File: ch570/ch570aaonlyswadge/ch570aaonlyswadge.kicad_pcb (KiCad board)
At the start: 2 copper layers, 42 x 26.8 mm, 53 parts, among them J1 SAO, J2 USB_C_Receptacle_USB2.0_16P, SW2 TS-1187A-B-A-B, U1 CH572D, U2 AW32001, U3 QMC6309, U4 USBLC6-2SC6, U7 MG6229D4-28, Y1 32MHz

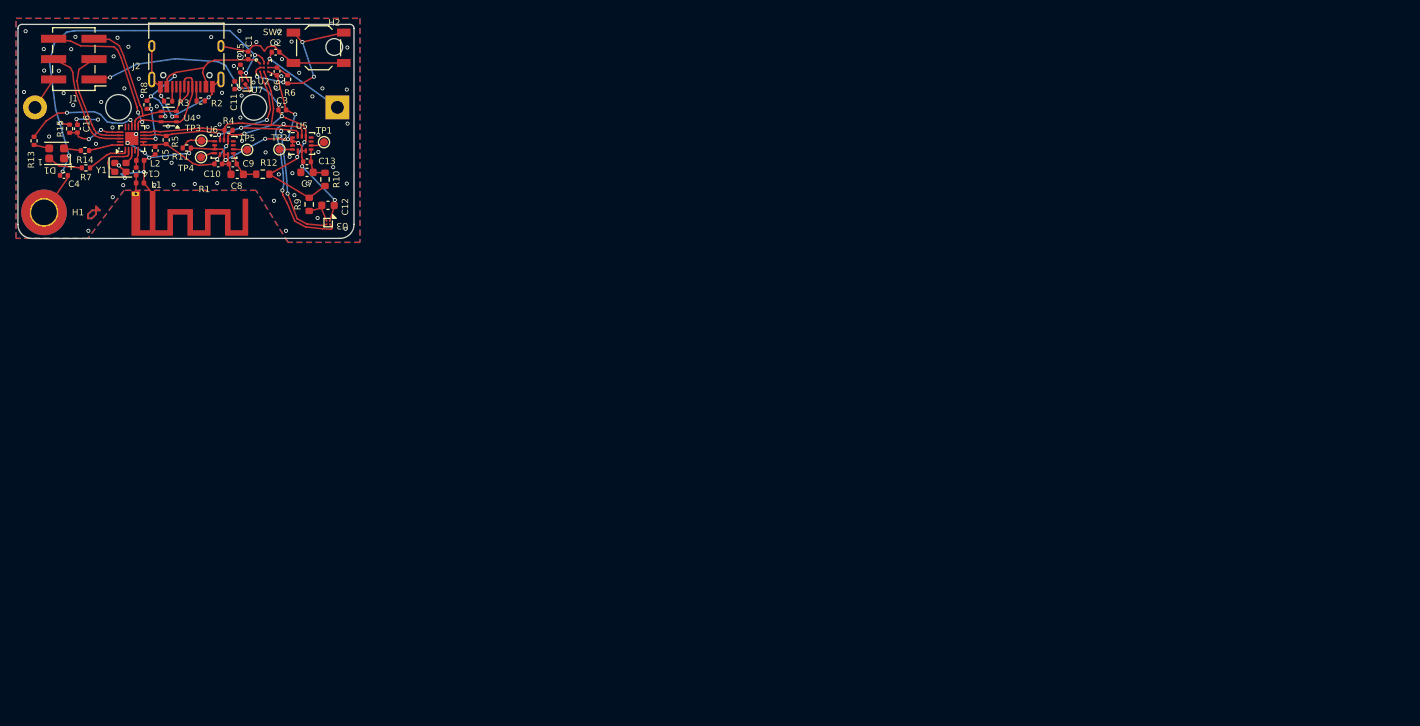
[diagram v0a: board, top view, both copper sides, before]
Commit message: Bump aa swadge
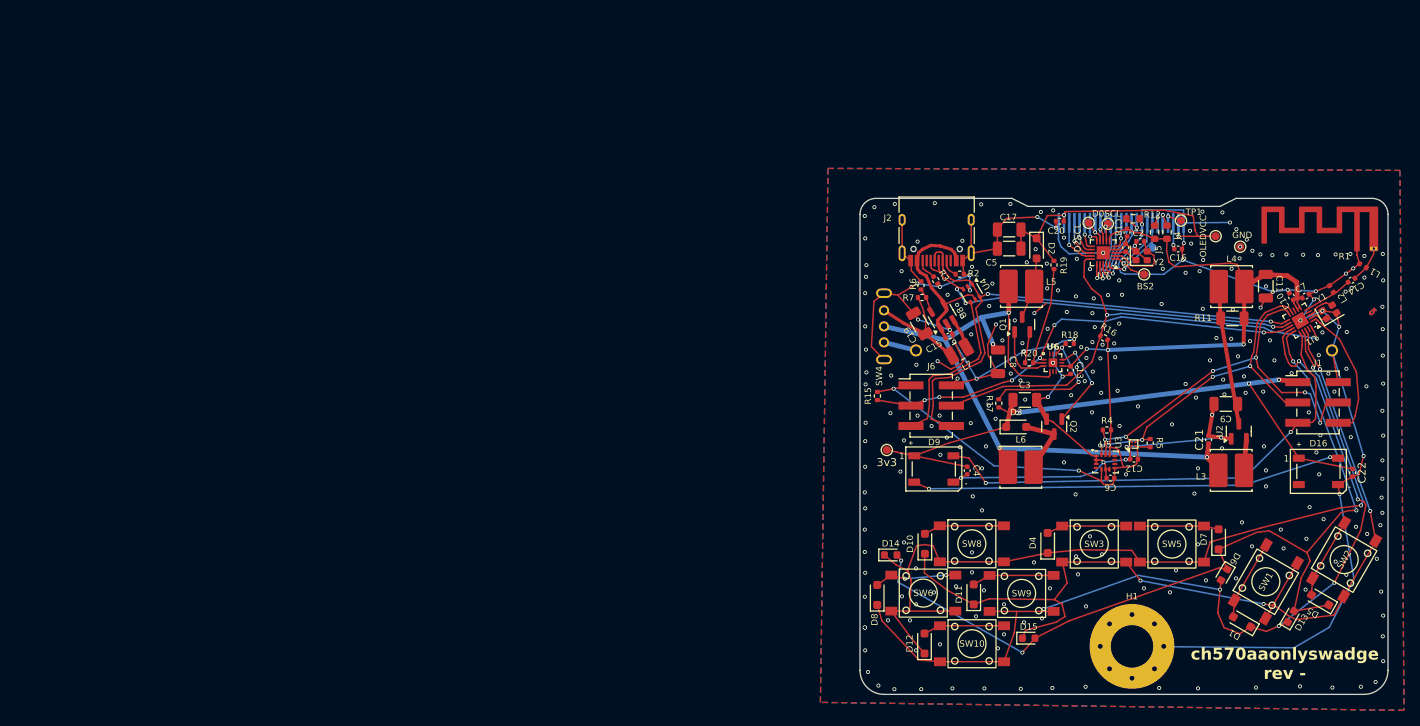
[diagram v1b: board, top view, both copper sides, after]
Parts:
- removed H2: BATTMOUNT, MountingHole:MountingHole_2.1mm
- removed R10, R9: 33Ω, Resistor_SMD:R_0603_1608Metric
- removed R13, R14: 1k, Resistor_SMD:R_0402_1005Metric
- removed R8: NP, Resistor_SMD:R_0402_1005Metric
- added C17: 22u25v-BASIC, Capacitor_SMD:C_1206_3216Metric, F.Cu at (187.7, 59.9)
- added C18: 1u, Capacitor_SMD:C_0402_1005Metric, F.Cu at (202.4, 60.3)
- added C19: 22u25v-BASIC, Capacitor_SMD:C_1206_3216Metric, F.Cu at (176.4, 71.6)
- added C20: 1u, Capacitor_SMD:C_0402_1005Metric, F.Cu at (194.0, 58.9)
- added C21: 1u, Capacitor_SMD:C_0402_1005Metric, F.Cu at (212.6, 86.2)
- added C22: 1u, Capacitor_SMD:C_0402_1005Metric, F.Cu at (230.6, 90.3)
- added D10: 1N4148WS, Diode_SMD:D_SOD-323_HandSoldering, F.Cu at (177.1, 99.2)
- added D11: 1N4148WS, Diode_SMD:D_SOD-323_HandSoldering, F.Cu at (183.2, 105.5)
- added D12: 1N4148WS, Diode_SMD:D_SOD-323_HandSoldering, F.Cu at (177.1, 111.6)
- added D13: RED, LED_SMD:LED_0603_1608Metric, F.Cu at (222.9, 108.3)
- added D14: RED, LED_SMD:LED_0603_1608Metric, F.Cu at (172.8, 100.6)
- added D15: RED, LED_SMD:LED_0603_1608Metric, F.Cu at (190.1, 111.0)
- added D16: WS2812B, LED_SMD:LED_WS2812B_PLCC4_5.0x5.0mm_P3.2mm, F.Cu at (226.3, 90.1)
- added D2: 1A-600mV, Diode_SMD:D_SOD-323_HandSoldering, F.Cu at (191.1, 62.2)
- added D3: 1A-600mV, Diode_SMD:D_SOD-323_HandSoldering, F.Cu at (188.5, 84.6)
- added D4: 1N4148WS, Diode_SMD:D_SOD-323_HandSoldering, F.Cu at (192.5, 99.1)
- added D5: 1N4148WS, Diode_SMD:D_SOD-323_HandSoldering, F.Cu at (226.5, 106.2)
- added D6: RED, LED_SMD:LED_0603_1608Metric, F.Cu at (214.5, 103.0)
- added D7: 1N4148WS, Diode_SMD:D_SOD-323_HandSoldering, F.Cu at (213.8, 98.6)
- added D8: 1N4148WS, Diode_SMD:D_SOD-323_HandSoldering, F.Cu at (171.2, 105.6)
- added D9: WS2812B, LED_SMD:LED_WS2812B_PLCC4_5.0x5.0mm_P3.2mm, F.Cu at (178.2, 89.8)
- added J3: OLED, cnhardware:RONBOE-OLED-25, B.Cu at (202.0, 59.1)
- added J4: J, Resistor_SMD:R_0603_1608Metric, F.Cu at (207.4, 60.2)
- added J5: J, Resistor_SMD:R_0603_1608Metric, F.Cu at (205.8, 60.2)
- added J6: PGM, Connector_PinHeader_2.54mm:PinHeader_2x03_P2.54mm_Vertical_SMD, F.Cu at (177.9, 81.9)
- added L3: 47uH 750mA 580mΩ, Inductor_SMD:L_Cenker_CKCS5020, F.Cu at (215.4, 90.0)
- added L4: 47uH 750mA 580mΩ, Inductor_SMD:L_Cenker_CKCS5020, F.Cu at (215.4, 67.0)
- added L5: 47uH 580mΩ, Inductor_SMD:L_Cenker_CKCS5020, F.Cu at (189.2, 67.0)
- added L6: 47uH 580mΩ, Inductor_SMD:L_Cenker_CKCS5020, F.Cu at (189.1, 89.6)
- added L7: 2.2uH, Inductor_SMD:L_1008_2520Metric, F.Cu at (181.3, 75.1)
- added Q1: 2300A, Package_TO_SOT_SMD:SOT-23, F.Cu at (189.3, 71.8)
- added Q2: 2300A, Package_TO_SOT_SMD:SOT-23, F.Cu at (193.3, 84.5)
- added R16: 5.1k, Resistor_SMD:R_0402_1005Metric, F.Cu at (199.5, 73.4)
- added R17: 5.1k, Resistor_SMD:R_0402_1005Metric, F.Cu at (186.3, 81.6)
- added R18: 5.1k, Resistor_SMD:R_0402_1005Metric, F.Cu at (195.2, 74.2)
- added R19: 51k, Resistor_SMD:R_0402_1005Metric, F.Cu at (193.2, 64.3)
- added R20: 5.1k, Resistor_SMD:R_0402_1005Metric, F.Cu at (190.1, 76.5)
- added SW1: YTS-D003-1A, cnhardware:YTS-D003-1A, F.Cu at (219.7, 103.9)
- added SW10: YTS-D003-1A, cnhardware:YTS-D003-1A, F.Cu at (183.0, 111.7)
- added SW3: YTS-D003-1A, cnhardware:YTS-D003-1A, F.Cu at (198.3, 99.2)
- added SW4: SW_SPDT_1825232-1, cnhardware:1825232-1, F.Cu at (172.0, 72.0)
- added SW5: YTS-D003-1A, cnhardware:YTS-D003-1A, F.Cu at (208.0, 99.2)
- added SW6: YTS-D003-1A, cnhardware:YTS-D003-1A, F.Cu at (176.9, 105.3)
- added SW8: YTS-D003-1A, cnhardware:YTS-D003-1A, F.Cu at (183.0, 99.2)
- added SW9: YTS-D003-1A, cnhardware:YTS-D003-1A, F.Cu at (189.2, 105.4)
- added TP6: OLEDVCC, TestPoint:TestPoint_Pad_D1.0mm, F.Cu at (213.4, 60.7)
- added TP7: GND, TestPoint:TestPoint_Pad_D1.0mm, F.Cu at (216.5, 62.0)
- added TP8: 3v3, TestPoint:TestPoint_Pad_D1.0mm, F.Cu at (172.3, 87.5)
- added U8: HX3406, Package_TO_SOT_SMD:SOT-23-5, F.Cu at (179.3, 70.7)
- added Y2: 24MHz, Crystal:Crystal_SMD_2016-4Pin_2.0x1.6mm, F.Cu at (204.2, 63.2)
- BT1: footprint Battery:BatteryHolder_Bulgin_BX0123_1xCR123 -> cnhardware:2460
- C1, C2: value 4.7u -> 10p
- C10, C13: value 0.1μF -> 1u
- C11, C9: value 0.1μF -> 100uF6.3v; footprint Capacitor_SMD:C_0402_1005Metric -> Capacitor_SMD:C_1206_3216Metric
- C12, C7: value 22μF -> 1u; footprint Capacitor_SMD:C_0603_1608Metric -> Capacitor_SMD:C_0402_1005Metric
- C15: value 1u -> 4.7u
- C16: value 0.1u -> 4.7u
- C3: value 4.7u -> 100uF6.3v; footprint Capacitor_SMD:C_0402_1005Metric -> Capacitor_SMD:C_1206_3216Metric
- C4: value 0.1u -> 1u
- C5: value 0.1u -> 22u25v-BASIC; footprint Capacitor_SMD:C_0402_1005Metric -> Capacitor_SMD:C_1206_3216Metric
- C8: value 22μF -> 100uF6.3v; footprint Capacitor_SMD:C_0603_1608Metric -> Capacitor_SMD:C_1206_3216Metric
- D1: value A-SP1923XR6GHB1C-M01-3T -> 1N4148WS; footprint LED_SMD:LED_RGB_Wuerth_150080M153000 -> Diode_SMD:D_SOD-323_HandSoldering
- H1: footprint MountingHole:MountingHole_3.2mm_M3_ISO7380_Pad_TopBottom -> MountingHole:MountingHole_5.3mm_M5_Pad_Via
- R11: value 5.1k -> J1; footprint Resistor_SMD:R_0402_1005Metric -> Resistor_SMD:R_1206_3216Metric
- R12: value 33Ω -> 1M
- R7: value 1k -> 5.1k
- SW2: value TS-1187A-B-A-B -> YTS-D003-1A; footprint Button_Switch_SMD:SW_SPST_TL3342 -> cnhardware:YTS-D003-1A
- TP1: value INT2 -> OLEDGPIO
- TP2: value INT1 -> BS1; moved to B.Cu
- TP3: value SA0 -> BS2
- TP4: value INT1 -> D0SCL
- TP5: value INT1 -> D2SCL
- U2: value AW32001 -> GR2188A22; footprint cnhardware:WLCSP-9-P0.5mm -> Package_TO_SOT_SMD:SOT-23
- U6: value ~ -> CH32V005D6U6; footprint cnhardware:LGA-14_3x2.5mm_P0.5mm_LayoutBorder3x4y_EVEN_PADS -> cnhardware:QFN-12-P0.4-WCH
- U7: value MG6229D4-28 -> CH32V006F8U6; footprint cnhardware:xdfn-reg -> Package_DFN_QFN:QFN-20-1EP_3x3mm_P0.4mm_EP1.65x1.65mm
- moved J1 161.3 mm to (226.2, 81.5), turned to 0 degrees
- moved D1 159.3 mm to (216.7, 108.9), turned to 150 degrees
- moved L1 153.2 mm to (231.9, 64.4), turned to 150 degrees
- moved C14 152.5 mm to (230.4, 66.2), turned to -150 degrees
- moved Y1 152.2 mm to (227.7, 70.2), turned to 30 degrees
- moved R1 150.7 mm to (231.1, 62.3), turned to 0 degrees
- moved L2 149.8 mm to (227.9, 67.3), turned to 120 degrees
- moved U1 147.8 mm to (224.0, 71.3), turned to -150 degrees
- moved H1 146.4 mm to (203.0, 112.0)
- moved SW2 143.3 mm to (229.5, 101.2), turned to 60 degrees
- moved C16 138.4 mm to (208.8, 62.3), turned to 0 degrees
- moved C10 135.2 mm to (222.9, 68.3), turned to 120 degrees
- moved R11 132.4 mm to (215.6, 71.0)
- moved C11 131.3 mm to (219.7, 67.0), turned to -90 degrees
- moved U2 130.1 mm to (216.3, 85.1), turned to 90 degrees
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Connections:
- BT1 pad 1: +BATT -> Net-(BT1-+)
- C1 pad 1: +5V -> Net-(U7-PA2)
- C10 pad 1: VDD -> +2V2
- C11 pad 1: VDD -> +2V2
- C12 pad 1: Net-(U3-VDD) -> +2V2
- C13 pad 1: Net-(U5-VDD) -> +2V2
- C15 pad 1: Net-(D1-A) (its old number) -> +5V
- C16 pad 1: LED -> Net-(J3-Pin_3)
- C2 pad 1: +BATT -> Net-(U7-PA1)
- C3 pad 1: VDD -> +3.3V
- C4 pad 1: Net-(D1-A) (its old number) -> +3.3V
- C5 pad 1: VDD -> OLEDVCC
- C6 pad 1: Net-(U2-VDD) -> +2V2
- C7 pad 1: Net-(U5-VDD) -> +2V2
- C8 pad 1: Net-(U6-VDD) -> +BATT
- C9 pad 1: Net-(U6-VDD) -> Net-(U2-OUT)
- D1 pad 1: Net-(D1-RK) -> CP_2
- J1 pad 1: VDD -> +3.3V
- J1 pad 3: PA10 -> SDA
- J1 pad 4: PA11 -> SCL
- J1 pad 5: SWCLK -> SAOGPIO1
- J1 pad 6: SWD -> SAOGPIO2
- R11 pad 1: Net-(U6-SD0/SA0) -> Net-(U2-OUT)
- R11 pad 2: GND -> +2V2
- R12 pad 1: Net-(U6-VDD) -> GND
- R12 pad 2: VDD -> Net-(J3-Pin_10)
- R15 pad 1: LED -> 005SWD
- R15 pad 2: Net-(D1-A) (its old number) -> +2V2
- R4 pad 2: VDD -> +2V2
- R5 pad 2: VDD -> +2V2
- R6 pad 1: PWRINT -> GND
- R6 pad 2: Net-(U2-VDD) -> Net-(U8-FB)
- R7 pad 1: PA3 -> Net-(U8-FB)
- R7 pad 2: Net-(D1-RK) -> USBBO
- SW2 pad 1: PWRINT -> Net-(D5-A)
- SW2 pad 2: GND -> Net-(D5-A)
- TP1 pad 1: Net-(U5-INT2) -> Net-(J3-Pin_4)
- TP2 pad 1: Net-(U5-INT1) -> OLEDBS1
- TP3 pad 1: Net-(U6-SD0/SA0) -> OLEDBS2
- TP4 pad 1: Net-(U6-INT1) -> D0SCL
- TP5 pad 1: Net-(U6-INT2) -> D2SCL
- U1 pad 1: PA3 -> SAOGPIO2
- U1 pad 13: PA4 -> 005SWD
- U1 pad 14: unconnected-(U1-PA5/SCK/SCL3-Pad14) -> CP_2
- U1 pad 15: unconnected-(U1-PA6/MISO/R4/SDA3-Pad15) -> CP_3
- U1 pad 16: LED -> SAOGPIO1
- U1 pad 17: PA10 -> CP_1
- U1 pad 18: PA11 -> CP_0
- U1 pad 20: PA2 -> 006SWD
- U1 pad 6: VDD -> +2V2
- U1 pad 7: VDD -> +2V2
- U1 pad 8: Net-(U1-V5) -> unconnected-(U1-V5-Pad8)
- U3 pad B1: Net-(U3-VDD) -> +2V2
- U5 pad 12: VDD -> +2V2
- U5 pad 4: Net-(U5-INT1) -> unconnected-(U5-INT1-Pad4)
- U5 pad 5: VDD -> +2V2
- U5 pad 8: Net-(U5-VDD) -> +2V2
- U5 pad 9: Net-(U5-INT2) -> unconnected-(U5-INT2-Pad9)
- U6 pad 1: Net-(U6-SD0/SA0) -> +BATT
- U6 pad 10: unconnected-(U6-CS-AUX-Pad10) -> 005SWD
- U6 pad 11: unconnected-(U6-SDO/A-Pad11) -> OLEDVMON
- U6 pad 12: VDD -> Net-(Q1-G)
- U6 pad 13: SCL -> GND
- U6 pad 2: GND -> unconnected-(U6-PA2/T1C2N/OPP0/XO/A0-Pad2)
- U6 pad 3: GND -> unconnected-(U6-PD0/T1C1N/SDA_/TX_/OPN1-Pad3)
- U6 pad 4: Net-(U6-INT1) -> +2V2
- U6 pad 5: VDD -> unconnected-(U6-PC0/T1C3_/T2C3-Pad5)
- U6 pad 6: GND -> Net-(Q2-G)
- U6 pad 7: GND -> 3V3MON
- U6 pad 8: Net-(U6-VDD) -> unconnected-(U6-PC6/T1C1_/T1C3N_-Pad8)
- U6 pad 9: Net-(U6-INT2) -> unconnected-(U6-PC7/T1C2_/T2C2_-Pad9)
- U7 pad 1: VDD -> OLEDBS2
- U7 pad 2: GND -> Net-(U7-PA1)
- U7 pad 3: Net-(D1-A) (its old number) -> Net-(U7-PA2)
- U7 pad 4: Net-(D1-A) (its old number) -> GND
- U7 pad 5: GND -> OLEDDC
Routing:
- net GND: track 117.6 -> 349.5 mm, vias 88 -> 284
- net +2V2: track 0.00 -> 130.7 mm, vias 0 -> 5
- net CP_2: track 0.00 -> 118.4 mm, vias 0 -> 6
- net CP_0: track 0.00 -> 117.0 mm, vias 0 -> 4
- net CP_1: track 0.00 -> 110.2 mm, vias 0 -> 2
- net CP_3: track 0.00 -> 109.9 mm, vias 0 -> 4
- net +3.3V: track 0.00 -> 81.7 mm, vias 0 -> 3
- net +BATT: track 11.9 -> 84.7 mm, vias 1 -> 4
- net VDD: track 72.5 -> 0.00 mm, vias 9 -> 0
- net 006SWD: track 0.00 -> 62.0 mm, vias 0 -> 2
- net SAOGPIO1: track 0.00 -> 61.3 mm, vias 0 -> 2
- net 005SWD: track 0.00 -> 57.1 mm, vias 0 -> 6
- net Net-(D16-DIN): track 0.00 -> 53.7 mm, vias 0 -> 2
- net Net-(D1-A) (its old number): track 52.7 -> 0.00 mm, vias 5 -> 0
- net SWCLK: track 24.6 -> 72.4 mm, vias 0 -> 3
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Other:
- board size 42 x 26.8 mm -> 66 x 62 mm
- board text added: "-"
- board text added: "ch570aaonlyswadge rev -"
- board text removed: "ch570cr123 - revA"
